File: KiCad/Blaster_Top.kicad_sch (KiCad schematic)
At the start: 13 parts, among them SW2 Fire, SW3 Freq Select, SW4 Fire Select, U3 Audio Board

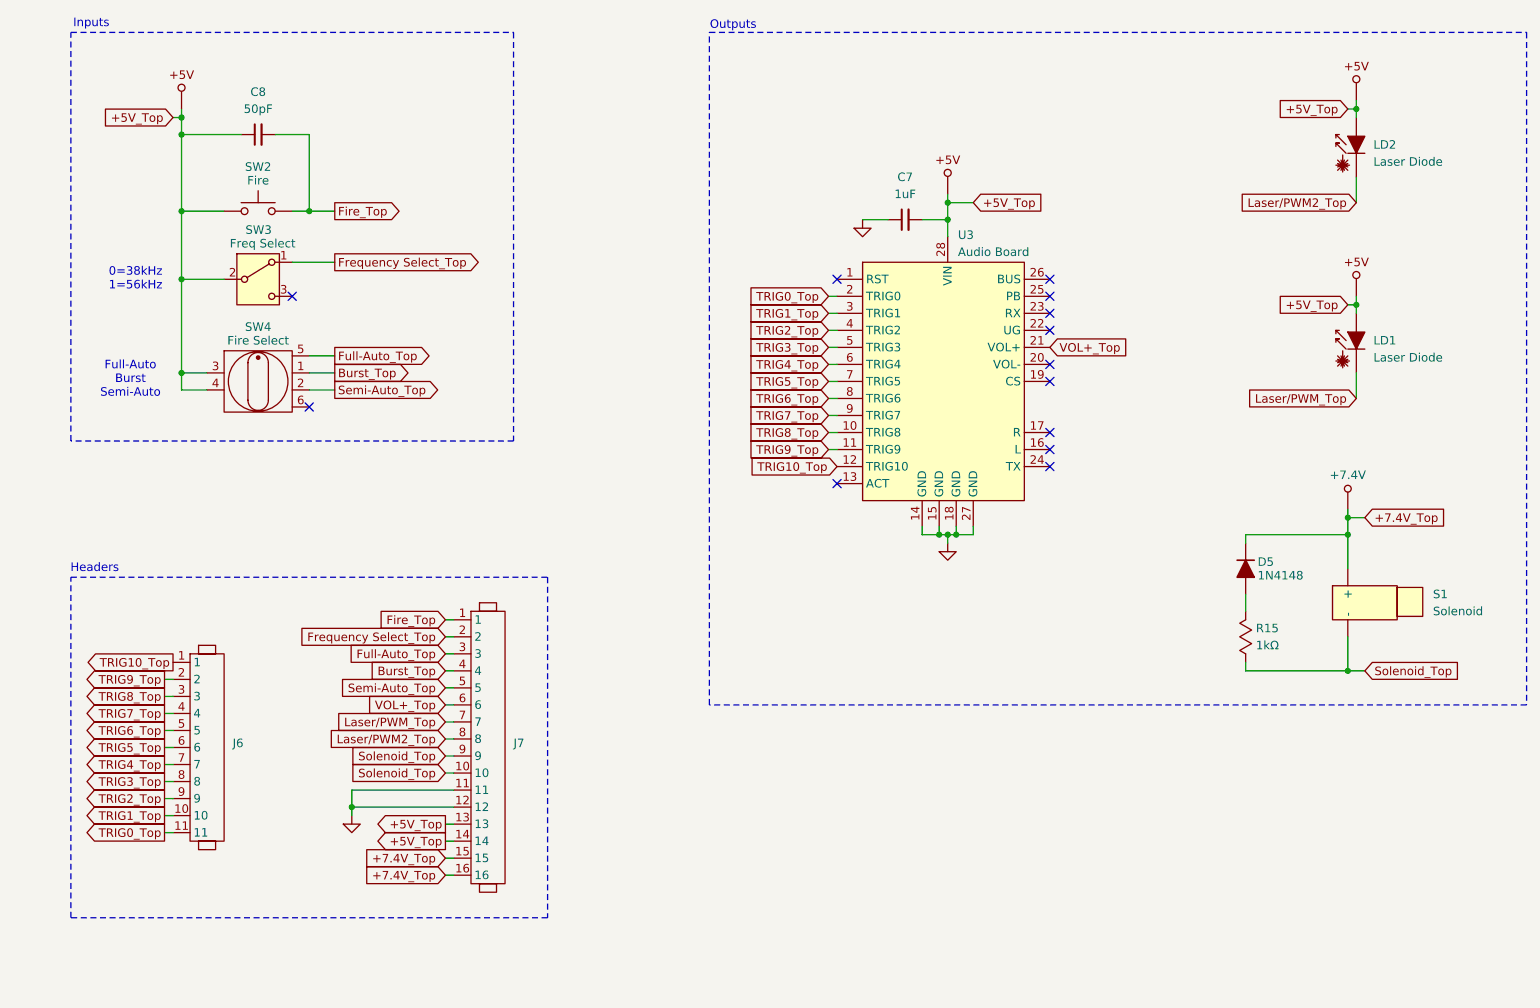
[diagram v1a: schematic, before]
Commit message: finished blaster PCB
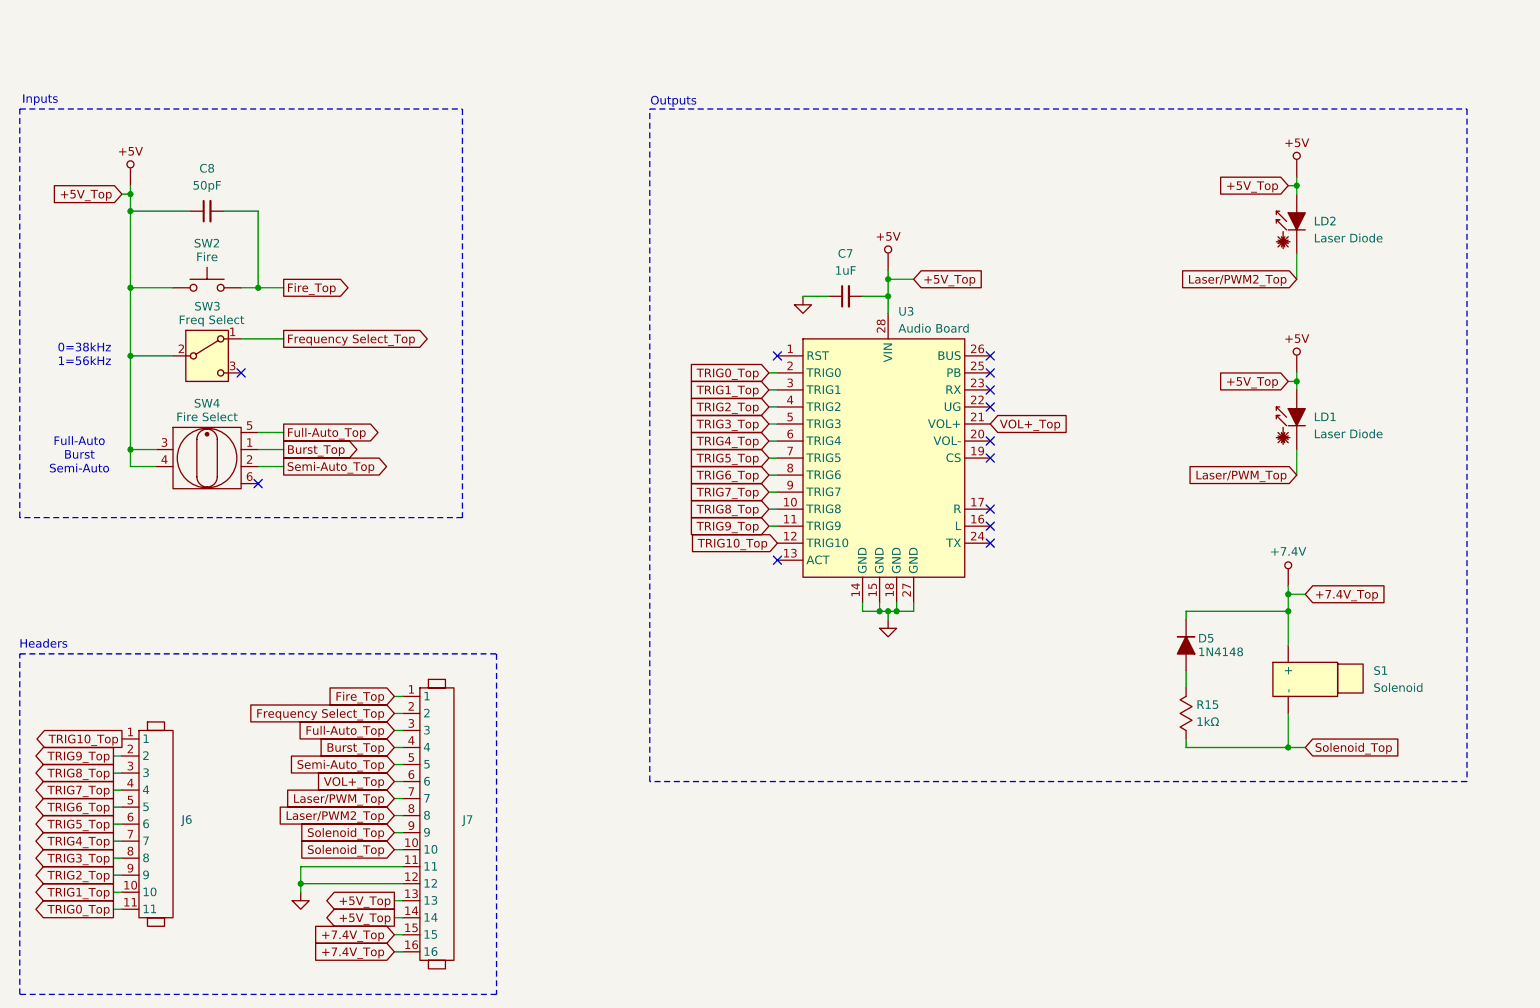
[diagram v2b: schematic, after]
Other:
- moved on the sheet: C7, C8, D5, J6, J7, LD1, LD2, R15, S1, SW2, SW3, SW4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
